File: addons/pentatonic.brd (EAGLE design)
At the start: 35.6 x 25.4 mm, 12 parts

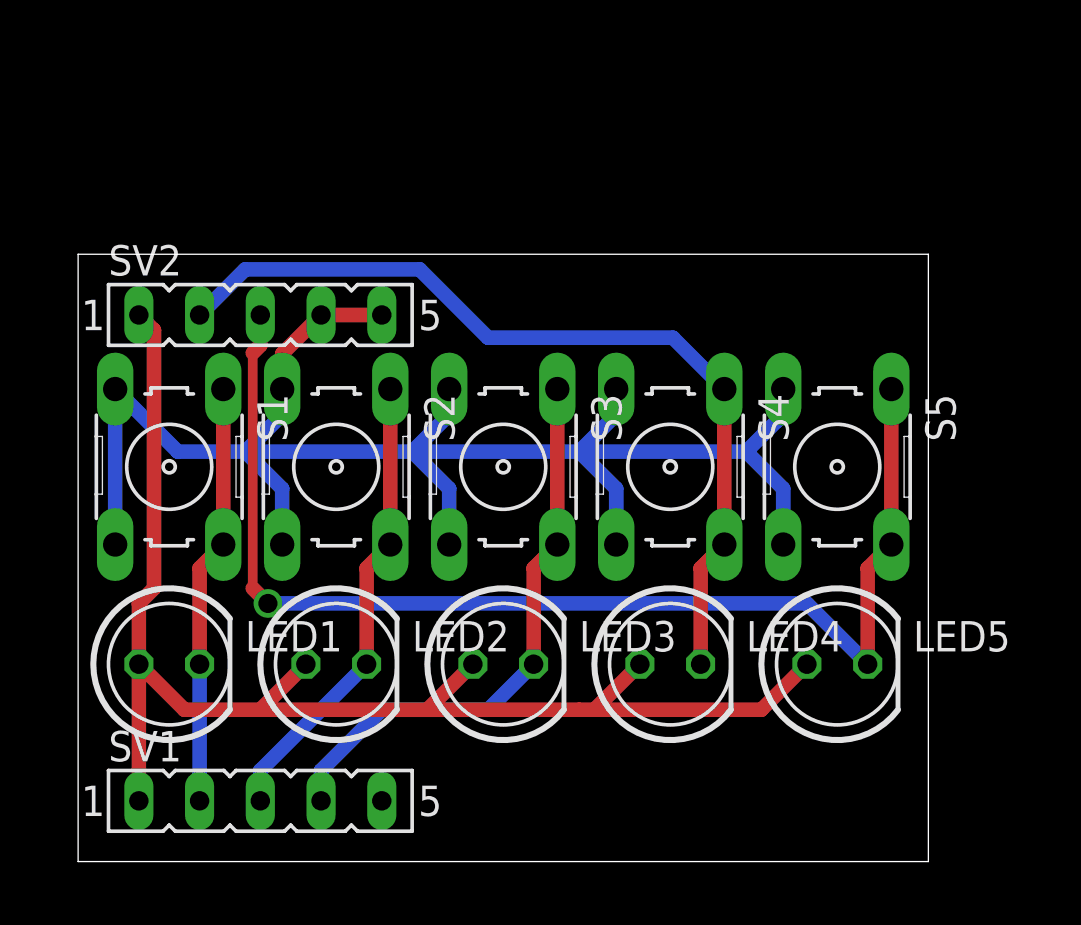
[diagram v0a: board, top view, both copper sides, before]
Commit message: anpassen an neues board
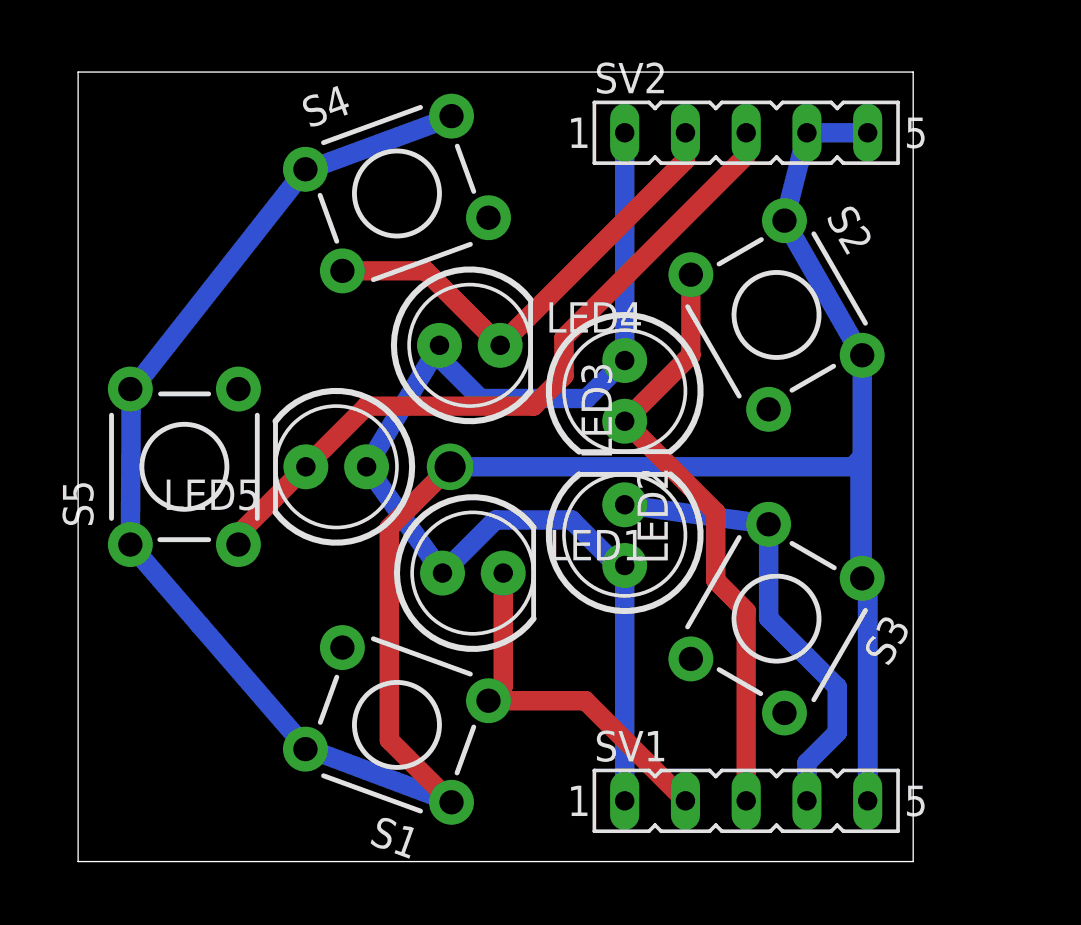
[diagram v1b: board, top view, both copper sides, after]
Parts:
- LED1, LED2, LED3, LED4, LED5: device led:LED5MM -> SparkFun:LED5MM
- S1, S2, S3, S4, S5: value (none) -> SWITCH-MOMENTARY-2PTH; device switch-omron:B3F-10XX -> SparkFun:TACTILE-PTH
- moved S5 27.3 mm to (4.45, 16.5), turned to 90 degrees
- moved LED5 22.5 mm to (10.8, 16.5), turned to 180 degrees
- moved SV2 21.7 mm to (27.9, 30.5)
- moved SV1 20.3 mm to (27.9, 2.54)
- moved S2 19.5 mm to (29.2, 22.9), turned to 300 degrees
- moved LED2 16.6 mm to (22.9, 19.7), turned to 270 degrees
- moved S4 16.2 mm to (13.3, 27.9), turned to 20 degrees
- moved LED4 15.8 mm to (16.4, 21.6)
- moved S1 14.4 mm to (13.3, 5.71), turned to 160 degrees
- moved LED1 13.3 mm to (16.5, 12.1)
- moved S3 13.1 mm to (29.2, 10.2), turned to 240 degrees
- moved LED3 7.41 mm to (22.9, 13.7), turned to 90 degrees
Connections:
- removed net PD2: LED1.K, S1.1, S1.2, SV1.2
- removed net PD3: LED2.K, S2.1, S2.2, SV1.3
- removed net PD4: LED3.K, S3.1, S3.2, SV1.4
- new net PB2: LED3.K, S3.3, SV1.4
- new net PC4: LED2.K, S2.3, SV1.3
- new net PC5: LED1.K, S1.3, SV1.2
- net GND: now also S1.1, S2.1, S3.1, S4.1, S5.1; no longer S1.3, S1.4, S2.3, S2.4, S3.3, S3.4, S4.3, S4.4, S5.3, S5.4
- net PD5: now also S4.3; no longer S4.1, S4.2
- net PD6: now also S5.3; no longer S5.1, S5.2
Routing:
- net GND: track 71.4 -> 115.4 mm, vias 0 -> 1
- net PC4: track 0.00 -> 25.3 mm
- net PD4: track 23.9 -> 0.00 mm
- net PD6: track 50.5 -> 30.1 mm, vias 1 -> 0
- net PD3: track 19.5 -> 0.00 mm
- net PB2: track 0.00 -> 19.4 mm
- net PD2: track 17.6 -> 0.00 mm
- net PD5: track 36.7 -> 20.0 mm
- net PC5: track 0.00 -> 15.6 mm
- net VCC: track 58.4 -> 49.7 mm
- net N$1: track 0.00 -> 6.43 mm
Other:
- board size 35.6 x 25.4 mm -> 34.9 x 33 mm
